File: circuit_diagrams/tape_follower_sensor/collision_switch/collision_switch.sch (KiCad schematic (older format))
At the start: 22 parts

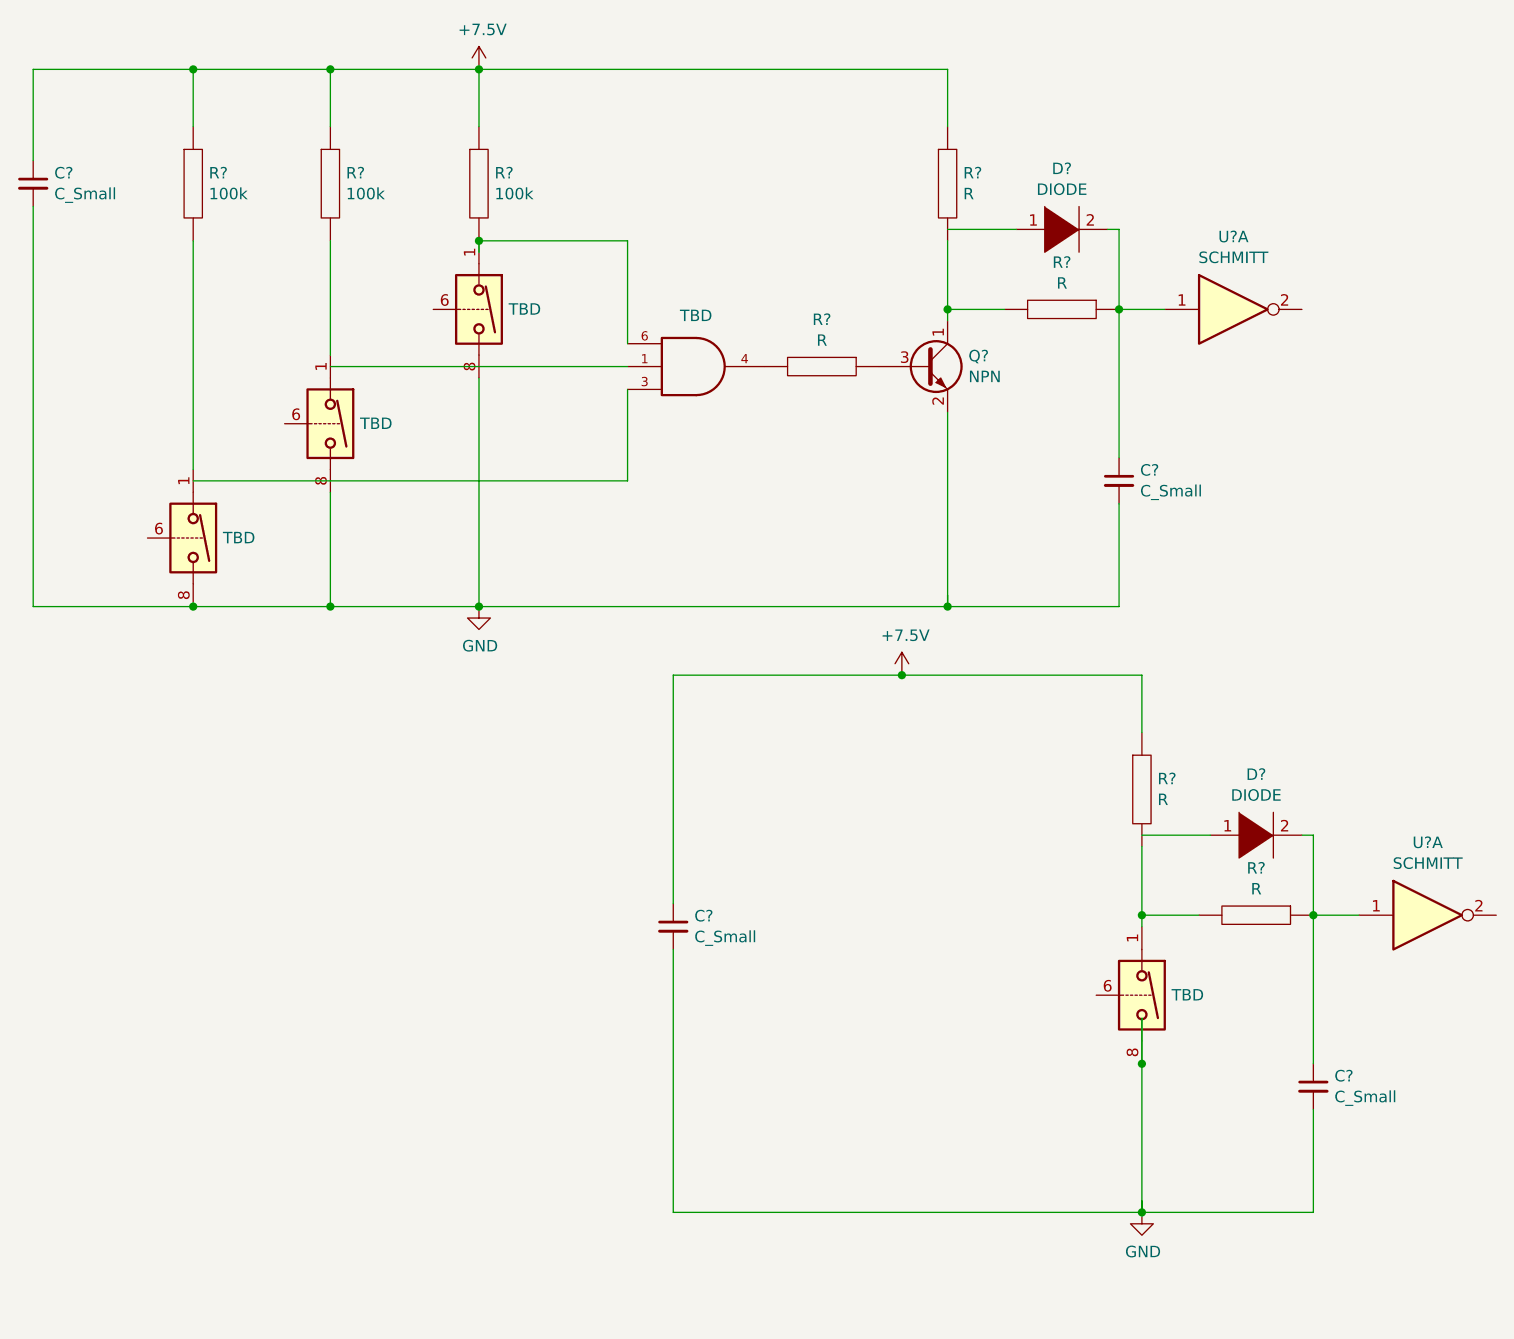
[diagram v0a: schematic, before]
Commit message: updated circuits and created pdfs
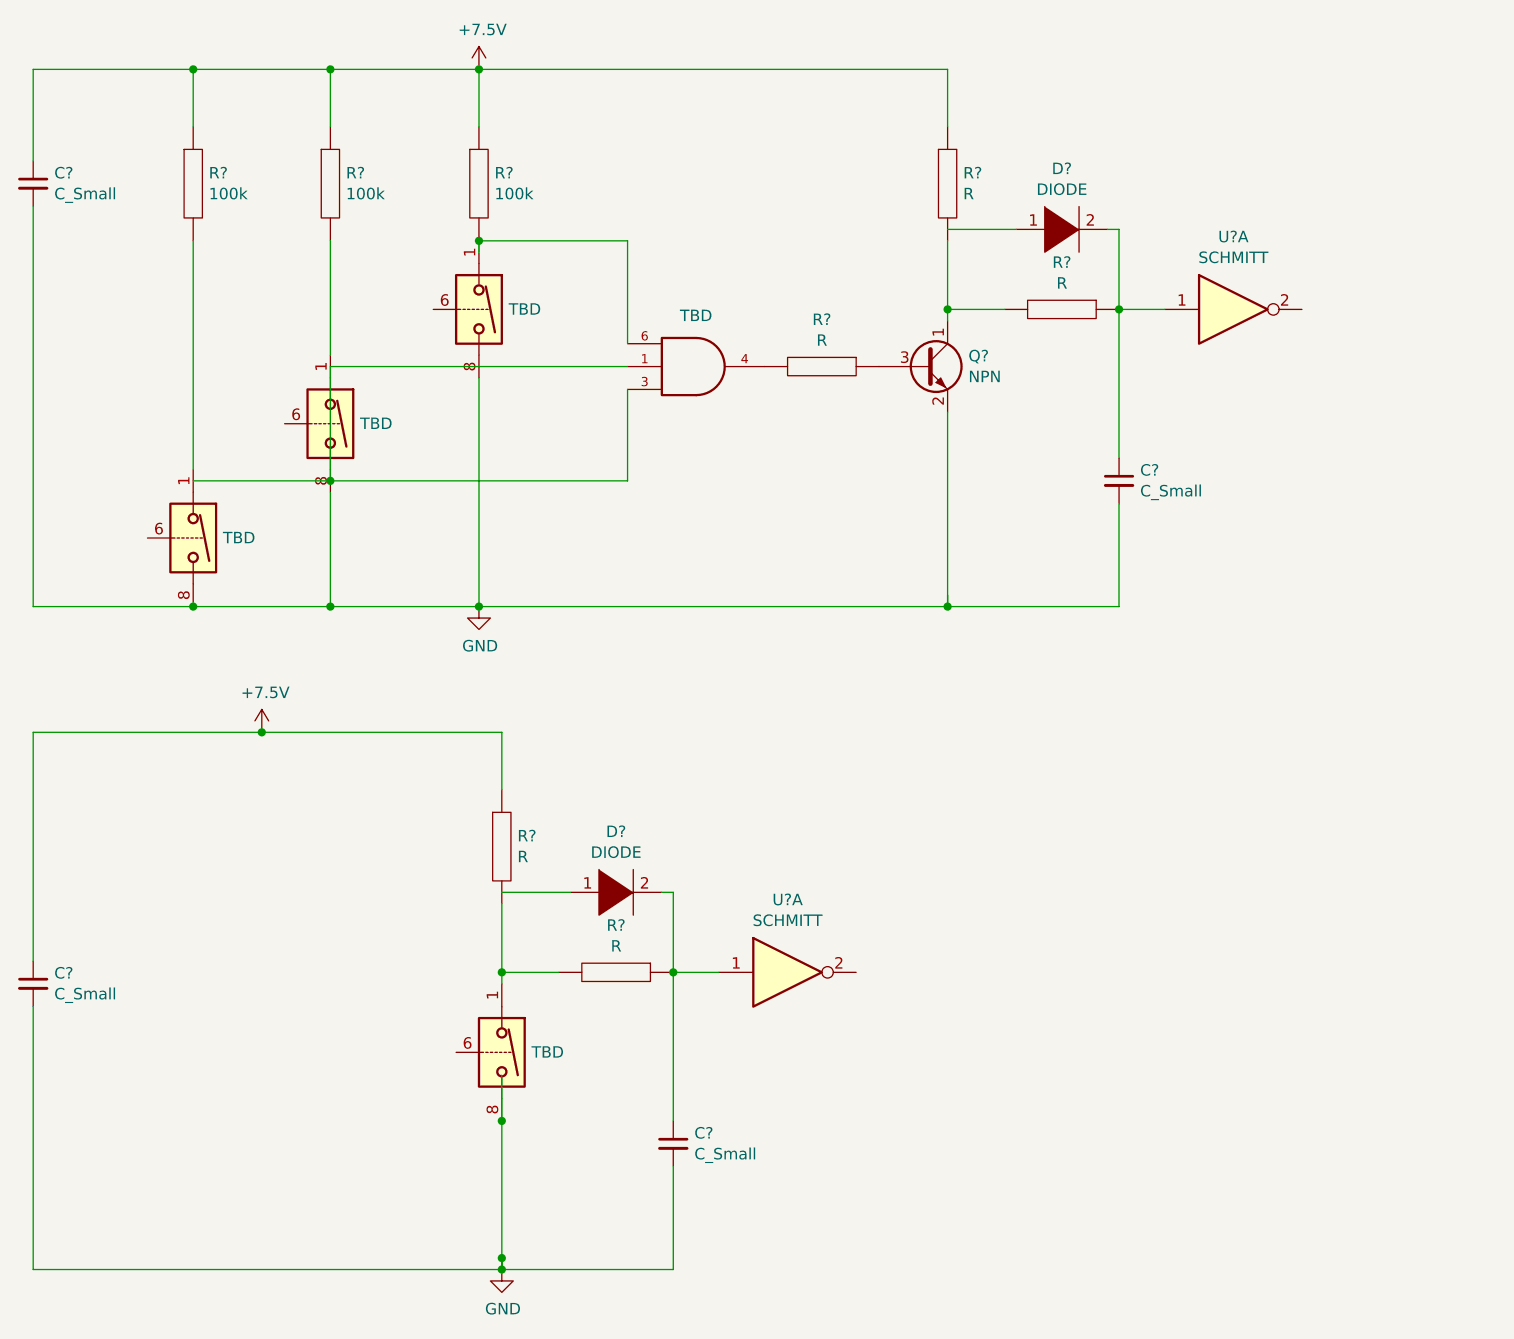
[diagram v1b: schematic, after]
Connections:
- wire segments 55 -> 57
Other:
- moved on the sheet: C?, D?, R?, U?A
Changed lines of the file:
@@
 EESchema Schematic File Version 4
+LIBS:collision_switch-cache
 EELAYER 29 0
 EELAYER END
@@
 	5650 2250 5650 2700
 Wire Wire Line
-	3750 3300 5650 3300
-Wire Wire Line
 	5650 3300 5650 2900
 $Comp
@@
 Connection ~ 7050 3850
 Wire Wire Line
-	5850 6500 7900 6500
+	3050 6750 5100 6750
 $Comp
 L pspice:R R?
 U 1 1 5D0233ED
-P 7900 4650
-F 0 "R?" H 7968 4696 50  0000 L CNN
-F 1 "R" H 7968 4605 50  0000 L CNN
-F 2 "" H 7900 4650 50  0001 C CNN
-F 3 "~" H 7900 4650 50  0001 C CNN
-	1    7900 4650
-	1    0    0    -1
-$EndComp
-Wire Wire Line
-	7900 4900 7900 5200
+P 5100 4900
+F 0 "R?" H 5168 4946 50  0000 L CNN
+F 1 "R" H 5168 4855 50  0000 L CNN
+F 2 "" H 5100 4900 50  0001 C CNN
+F 3 "~" H 5100 4900 50  0001 C CNN
+	1    5100 4900
+	1    0    0    -1
+$EndComp
+Wire Wire Line
+	5100 5150 5100 5450
 $Comp
 L pspice:R R?
 U 1 1 5D0233F4
-P 8400 5200
-F 0 "R?" V 8195 5200 50  0000 C CNN
-F 1 "R" V 8286 5200 50  0000 C CNN
-F 2 "" H 8400 5200 50  0001 C CNN
-F 3 "~" H 8400 5200 50  0001 C CNN
-	1    8400 5200
+P 5600 5450
+F 0 "R?" V 5395 5450 50  0000 C CNN
+F 1 "R" V 5486 5450 50  0000 C CNN
+F 2 "" H 5600 5450 50  0001 C CNN
+F 3 "~" H 5600 5450 50  0001 C CNN
+	1    5600 5450
 	0    1    1    0
 $EndComp
@@
 L pspice:DIODE D?
 U 1 1 5D0233FA
-P 8400 4850
-F 0 "D?" H 8400 5115 50  0000 C CNN
-F 1 "DIODE" H 8400 5024 50  0000 C CNN
-F 2 "" H 8400 4850 50  0001 C CNN
-F 3 "~" H 8400 4850 50  0001 C CNN
-	1    8400 4850
+P 5600 5100
+F 0 "D?" H 5600 5365 50  0000 C CNN
+F 1 "DIODE" H 5600 5274 50  0000 C CNN
+F 2 "" H 5600 5100 50  0001 C CNN
+F 3 "~" H 5600 5100 50  0001 C CNN
+	1    5600 5100
 	1    0    0    -1
 $EndComp
@@
 L Device:C_Small C?
 U 1 1 5D023400
-P 8650 5950
-F 0 "C?" H 8742 5996 50  0000 L CNN
-F 1 "C_Small" H 8742 5905 50  0000 L CNN
-F 2 "" H 8650 5950 50  0001 C CNN
-F 3 "~" H 8650 5950 50  0001 C CNN
-	1    8650 5950
+P 5850 6200
+F 0 "C?" H 5942 6246 50  0000 L CNN
+F 1 "C_Small" H 5942 6155 50  0000 L CNN
+F 2 "" H 5850 6200 50  0001 C CNN
+F 3 "~" H 5850 6200 50  0001 C CNN
+	1    5850 6200
 	1    0    0    -1
 $EndComp
@@
 L 74xx:74HC14 U?
 U 1 1 5D023406
-P 9150 5200
-F 0 "U?" H 9150 5517 50  0000 C CNN
-F 1 "SCHMITT" H 9150 5426 50  0000 C CNN
-F 2 "" H 9150 5200 50  0001 C CNN
-F 3 "http://www.ti.com/lit/gpn/sn74HC14" H 9150 5200 50  0001 C CNN
-	1    9150 5200
-	1    0    0    -1
-$EndComp
-Wire Wire Line
-	5850 4150 6850 4150
-Wire Wire Line
-	7900 4150 7900 4400
-Wire Wire Line
-	7900 4850 8200 4850
-Wire Wire Line
-	7900 5200 8150 5200
-Connection ~ 7900 5200
-Wire Wire Line
-	7900 5200 7900 5250
-Wire Wire Line
-	8600 4850 8650 4850
-Wire Wire Line
-	8650 4850 8650 5200
-Wire Wire Line
-	8850 5200 8650 5200
-Connection ~ 8650 5200
-Wire Wire Line
-	8650 5200 8650 5850
-Wire Wire Line
-	8650 6050 8650 6500
-Wire Wire Line
-	8650 6500 7900 6500
-Connection ~ 7900 6500
+P 6350 5450
+F 0 "U?" H 6350 5767 50  0000 C CNN
+F 1 "SCHMITT" H 6350 5676 50  0000 C CNN
+F 2 "" H 6350 5450 50  0001 C CNN
+F 3 "http://www.ti.com/lit/gpn/sn74HC14" H 6350 5450 50  0001 C CNN
+	1    6350 5450
+	1    0    0    -1
+$EndComp
+Wire Wire Line
+	3050 4400 4050 4400
+Wire Wire Line
+	5100 4400 5100 4650
+Wire Wire Line
+	5100 5100 5400 5100
+Wire Wire Line
+	5100 5450 5350 5450
+Connection ~ 5100 5450
+Wire Wire Line
+	5100 5450 5100 5500
+Wire Wire Line
+	5800 5100 5850 5100
+Wire Wire Line
+	5850 5100 5850 5450
+Wire Wire Line
+	6050 5450 5850 5450
+Connection ~ 5850 5450
+Wire Wire Line
+	5850 5450 5850 6100
+Wire Wire Line
+	5850 6300 5850 6750
+Wire Wire Line
+	5850 6750 5100 6750
+Connection ~ 5100 6750
 Wire Wire Line
 	7050 3800 7050 3850
 Wire Wire Line
-	7900 6450 7900 6500
-Wire Wire Line
 	7050 3000 7050 3850
 Wire Wire Line
-	7900 5650 7900 5850
+	5100 5900 5100 6100
 $Comp
 L Analog_Switch:ADG417BN U?
 U 1 1 5D0249FC
-P 7900 5550
-F 0 "U?" V 7854 5680 50  0001 L CNN
-F 1 "TBD" V 7900 5680 50  0000 L CNN
-F 2 "Package_DIP:DIP-8_W7.62mm" H 7900 5450 50  0001 C CNN
-F 3 "https://www.analog.com/media/en/technical-documentation/data-sheets/ADG417.pdf" H 7900 5550 50  0001 C CNN
-	1    7900 5550
-	0    1    1    0
-$EndComp
-Connection ~ 7900 5850
-Wire Wire Line
-	7900 5850 7900 6500
+P 5100 5800
+F 0 "U?" V 5054 5930 50  0001 L CNN
+F 1 "TBD" V 5100 5930 50  0000 L CNN
+F 2 "Package_DIP:DIP-8_W7.62mm" H 5100 5700 50  0001 C CNN
+F 3 "https://www.analog.com/media/en/technical-documentation/data-sheets/ADG417.pdf" H 5100 5800 50  0001 C CNN
+	1    5100 5800
+	0    1    1    0
+$EndComp
+Connection ~ 5100 6100
 $Comp
 L Device:C_Small C?
 U 1 1 5D026393
-P 5850 5250
-F 0 "C?" H 5942 5296 50  0000 L CNN
-F 1 "C_Small" H 5942 5205 50  0000 L CNN
-F 2 "" H 5850 5250 50  0001 C CNN
-F 3 "~" H 5850 5250 50  0001 C CNN
-	1    5850 5250
-	1    0    0    -1
-$EndComp
-Wire Wire Line
-	5850 4150 5850 5150
-Wire Wire Line
-	5850 5350 5850 6500
+P 3050 5500
+F 0 "C?" H 3142 5546 50  0000 L CNN
+F 1 "C_Small" H 3142 5455 50  0000 L CNN
+F 2 "" H 3050 5500 50  0001 C CNN
+F 3 "~" H 3050 5500 50  0001 C CNN
+	1    3050 5500
+	1    0    0    -1
+$EndComp
+Wire Wire Line
+	3050 4400 3050 5400
+Wire Wire Line
+	3050 5600 3050 6750
 $Comp
 L power:GND #PWR?
@@
 L power:GND #PWR?
 U 1 1 5D028E6B
-P 7900 6500
-F 0 "#PWR?" H 7900 6250 50  0001 C CNN
-F 1 "GND" H 7905 6327 50  0000 C CNN
-F 2 "" H 7900 6500 50  0001 C CNN
-F 3 "" H 7900 6500 50  0001 C CNN
-	1    7900 6500
+P 5100 6750
+F 0 "#PWR?" H 5100 6500 50  0001 C CNN
+F 1 "GND" H 5105 6577 50  0000 C CNN
+F 2 "" H 5100 6750 50  0001 C CNN
+F 3 "" H 5100 6750 50  0001 C CNN
+	1    5100 6750
 	1    0    0    -1
 $EndComp
@@
 L power:+7.5V #PWR?
 U 1 1 5D029628
-P 6850 4150
-F 0 "#PWR?" H 6850 4000 50  0001 C CNN
-F 1 "+7.5V" H 6865 4323 50  0000 C CNN
-F 2 "" H 6850 4150 50  0001 C CNN
-F 3 "" H 6850 4150 50  0001 C CNN
-	1    6850 4150
-	1    0    0    -1
-$EndComp
-Connection ~ 6850 4150
-Wire Wire Line
-	6850 4150 7900 4150
+P 4050 4400
+F 0 "#PWR?" H 4050 4250 50  0001 C CNN
+F 1 "+7.5V" H 4065 4573 50  0000 C CNN
+F 2 "" H 4050 4400 50  0001 C CNN
+F 3 "" H 4050 4400 50  0001 C CNN
+	1    4050 4400
+	1    0    0    -1
+$EndComp
+Connection ~ 4050 4400
+Wire Wire Line
+	4050 4400 5100 4400
+Wire Wire Line
+	4350 3300 4350 2800
+Wire Wire Line
+	3750 3300 4350 3300
+Connection ~ 4350 3300
+Wire Wire Line
+	4350 3300 5650 3300
+Connection ~ 5100 6700
+Wire Wire Line
+	5100 6700 5100 6750
+Wire Wire Line
+	5100 6100 5100 6750
 $EndSCHEMATC
